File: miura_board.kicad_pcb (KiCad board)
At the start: 2 copper layers, 73.5 x 56.8 mm, 22 parts, among them J1 Conn_01x02_Female, SW1 SW_Push, U1 ATmega32U4-A, U2 NRF24L01, Y1 16MHz, Y2 16MHz

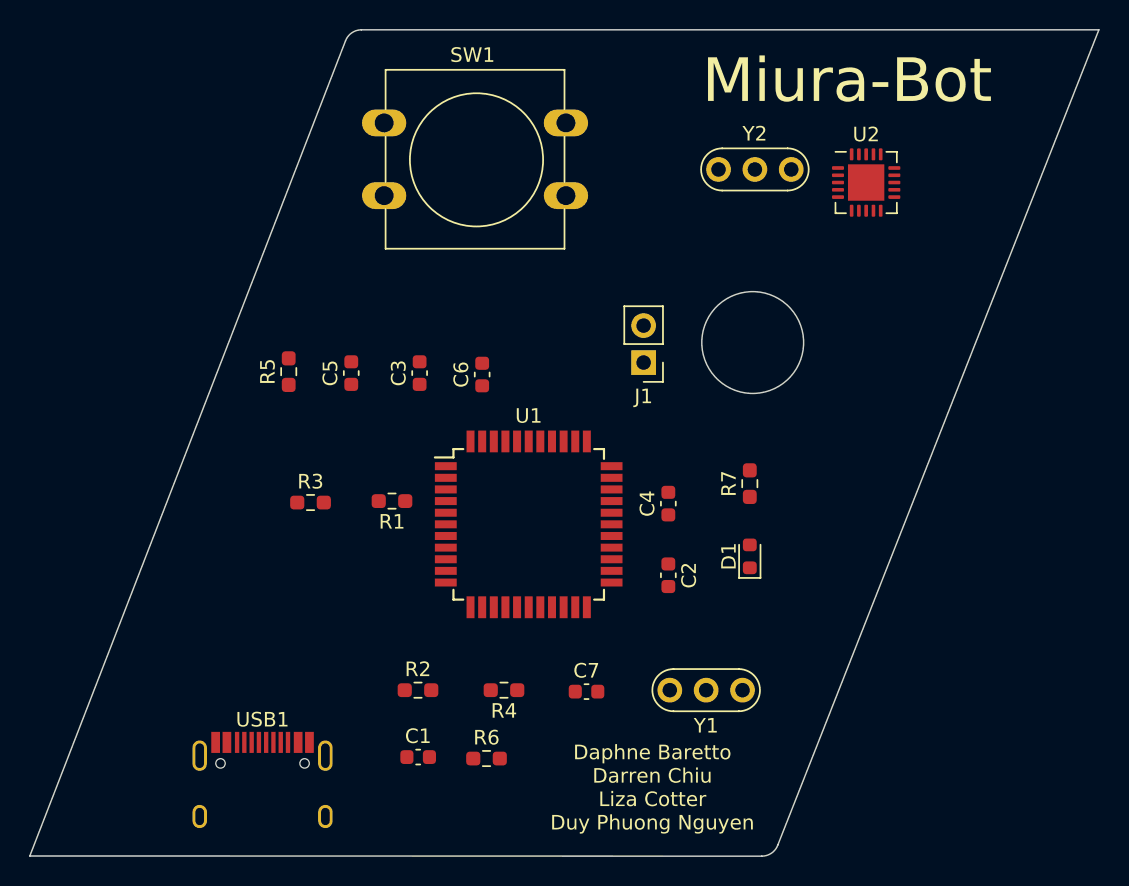
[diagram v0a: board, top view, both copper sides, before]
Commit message: Corners
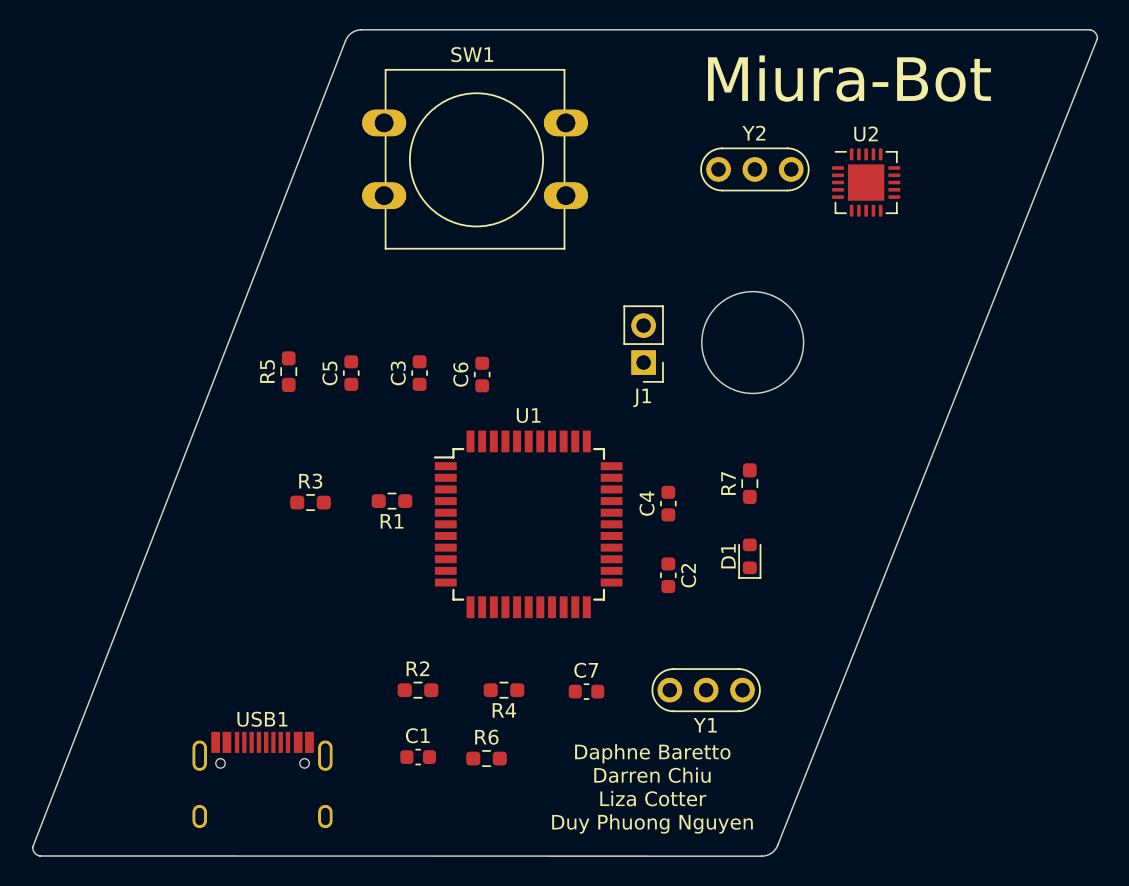
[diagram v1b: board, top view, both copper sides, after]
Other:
- board size 73.5 x 56.8 mm -> 73.2 x 56.8 mm
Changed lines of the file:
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@@
   )
   (gr_arc (start 73.100001 24.970469) (mid 73.528537 24.41182) (end 74.2 24.2) (layer "Edge.Cuts") (width 0.1))
+  (gr_arc (start 124.3 24.2) (mid 124.661364 24.407196) (end 124.8 24.8) (layer "Edge.Cuts") (width 0.1))
+  (gr_arc (start 52.1 81) (mid 51.738636 80.792804) (end 51.6 80.4) (layer "Edge.Cuts") (width 0.1))
   (gr_arc (start 102.828504 80.241307) (mid 102.4 80.8) (end 101.728505 81.011776) (layer "Edge.Cuts") (width 0.1))
-  (gr_line (start 102.828504 80.241307) (end 124.9 24.2) (layer "Edge.Cuts") (width 0.1))
-  (gr_line (start 51.4 81) (end 101.728505 81.011776) (layer "Edge.Cuts") (width 0.1))
-  (gr_line (start 51.4 81) (end 73.100001 24.970469) (layer "Edge.Cuts") (width 0.1))
-  (gr_line (start 74.2 24.2) (end 124.9 24.2) (layer "Edge.Cuts") (width 0.1))
+  (gr_line (start 102.828504 80.241307) (end 124.8 24.8) (layer "Edge.Cuts") (width 0.1))
+  (gr_line (start 52.1 81) (end 101.728505 81.011776) (layer "Edge.Cuts") (width 0.1))
+  (gr_line (start 51.6 80.4) (end 73.100001 24.970469) (layer "Edge.Cuts") (width 0.1))
+  (gr_line (start 74.2 24.2) (end 124.3 24.2) (layer "Edge.Cuts") (width 0.1))
   (gr_circle (center 101.1 45.7) (end 104.6 45.7) (layer "Edge.Cuts") (width 0.1) (fill none))
   (gr_text "Miura-Bot\n" (at 107.6 27.7) (layer "F.SilkS")
